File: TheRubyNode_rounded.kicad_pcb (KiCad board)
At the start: 2 copper layers, 141 x 79.5 mm, 66 parts, among them J1 USB4085-GF-A_REVB, J2 Conn_02x01, J3 Conn_02x01, J4 Conn_01x02, J5 91930-21111LF, J6 Conn_01x04, J7 Conn_01x03, J8 Conn_02x01, Q1 Si2307, SW1 SW_SPST, SW2 SW_Push, SW3 SW_Push, SW4 SW_Push, U1 INA219AxD, U2 LoRa1121F33-2G4, U3 SC189Z, U4 MCP73833-AMI-UN, U5 ESP32-S3-WROOM-1, U6 USBLC6-2SC6, U7 ISL97519A

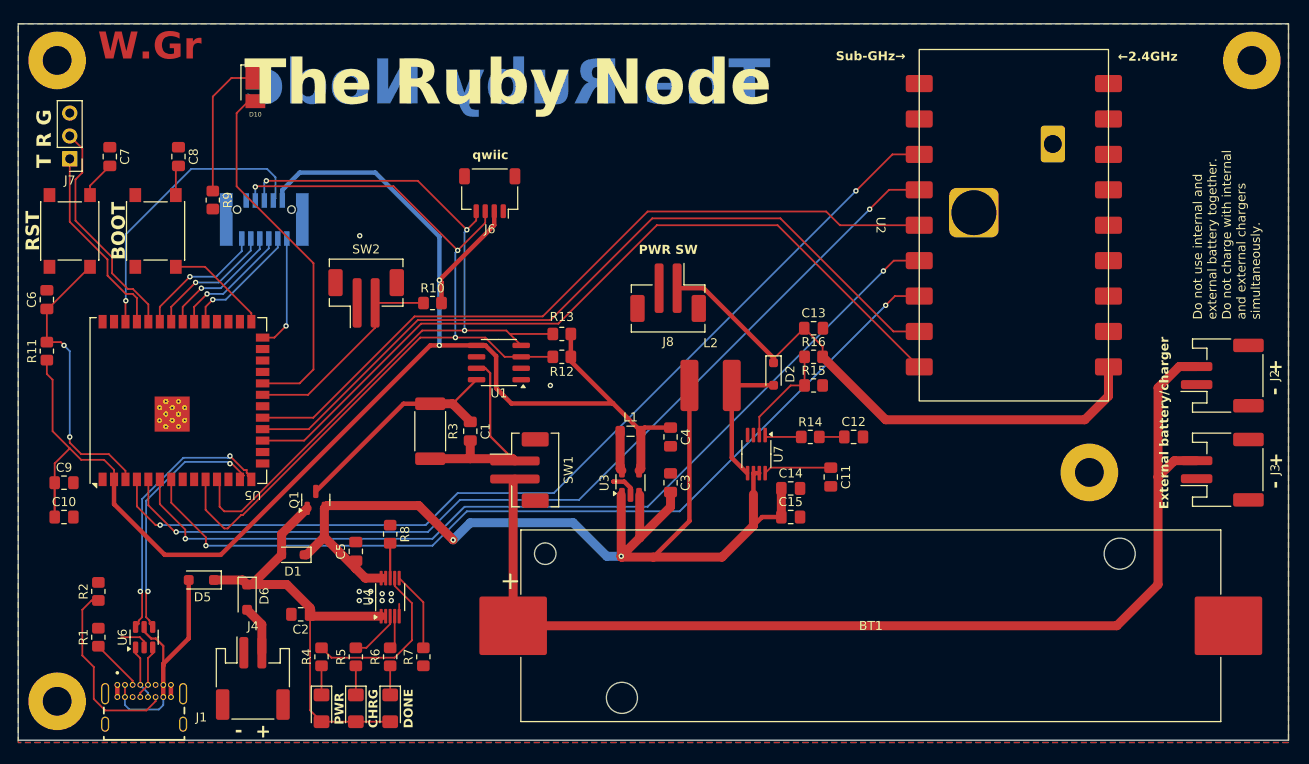
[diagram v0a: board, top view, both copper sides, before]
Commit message: Add PCB design
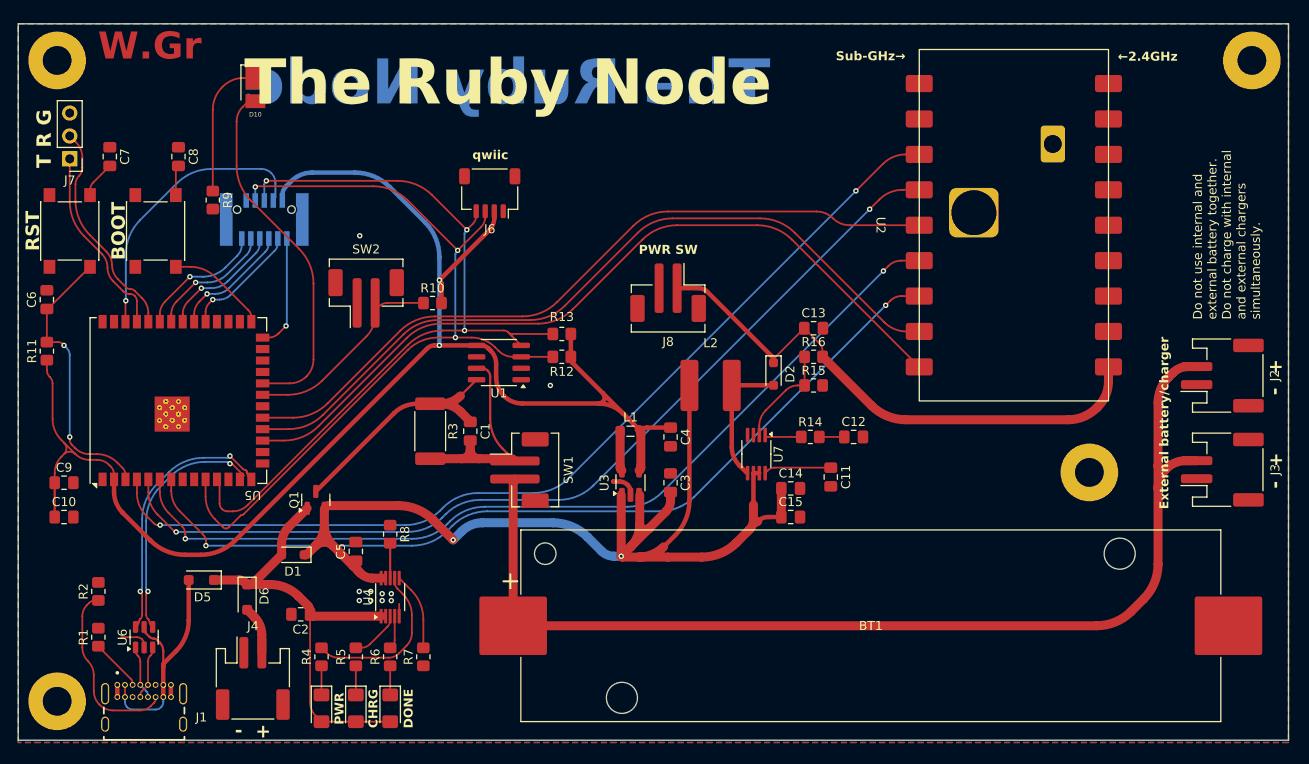
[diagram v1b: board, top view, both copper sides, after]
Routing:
- net +BATT: track 123.3 -> 132.4 mm
- net +3V3: track 170.6 -> 173.5 mm
- net Net-(Q1-D): track 25.8 -> 28.5 mm
- net LR_RST: track 87.8 -> 86.3 mm
- net Net-(SW1-A): track 24.1 -> 25.5 mm
- net Net-(BT1-+): track 122.0 -> 123.3 mm
- net LR_IRQ: track 89.3 -> 88.0 mm
- net LR_BUSY: track 83.0 -> 81.7 mm
- net +5V: track 62.6 -> 61.4 mm
- net SPI_SCK: track 107.7 -> 106.6 mm
- net LR_CS: track 105.5 -> 104.4 mm
- net I2C_SDA: track 94.4 -> 93.3 mm
- net SPI_MOSI: track 101.7 -> 100.6 mm
- net SPI_MISO: track 99.6 -> 98.5 mm
- net Net-(U5-IO13): track 23.7 -> 22.6 mm
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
